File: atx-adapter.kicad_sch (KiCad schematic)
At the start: 1 part

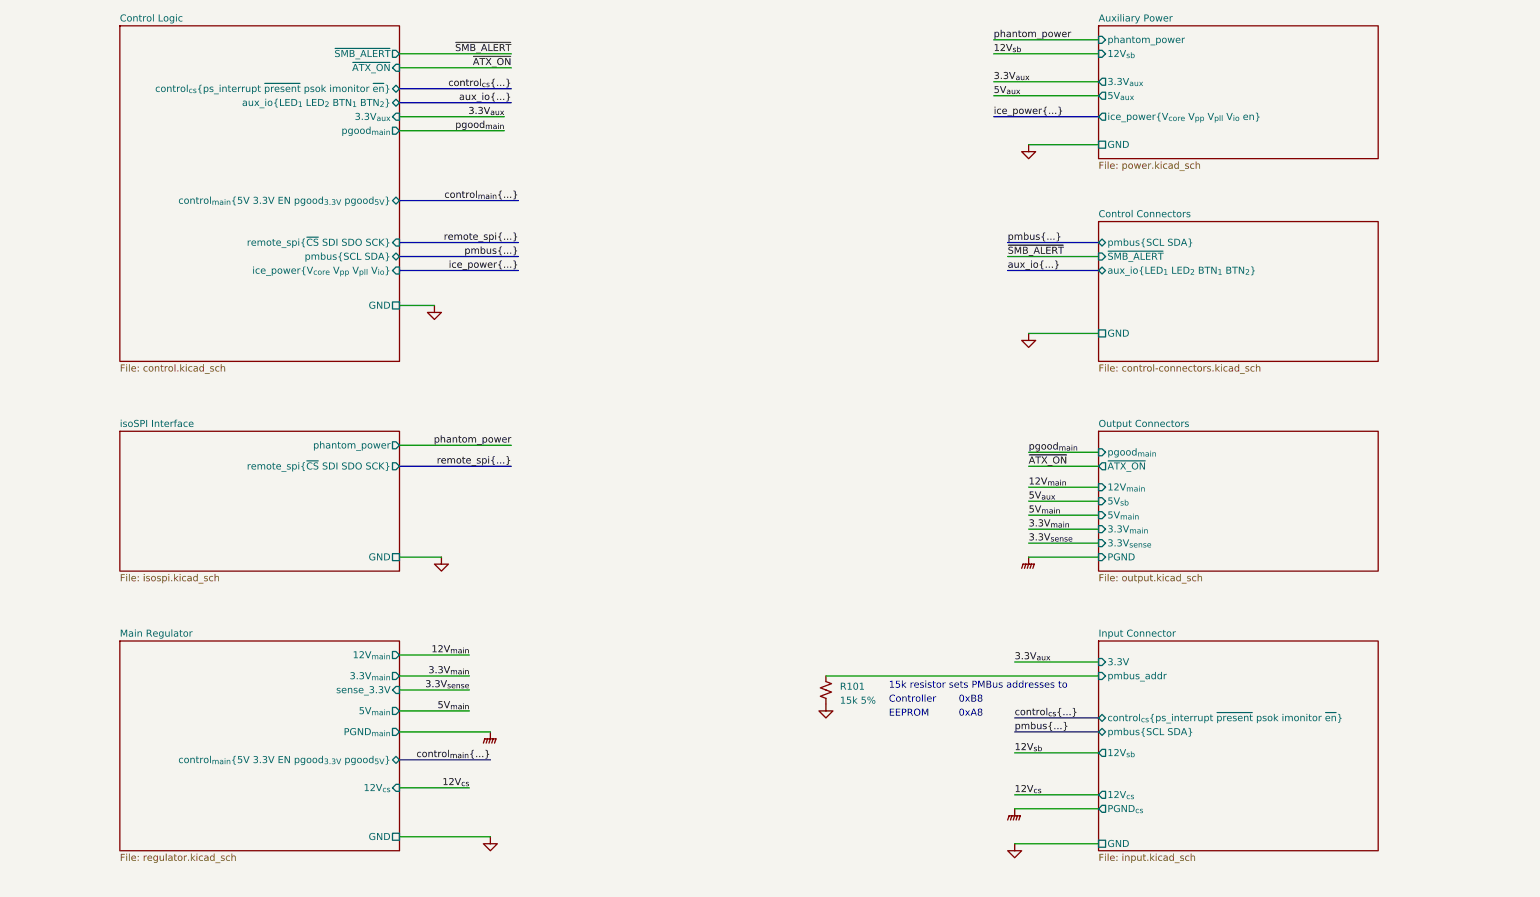
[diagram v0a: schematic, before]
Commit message: flesh out remote interface
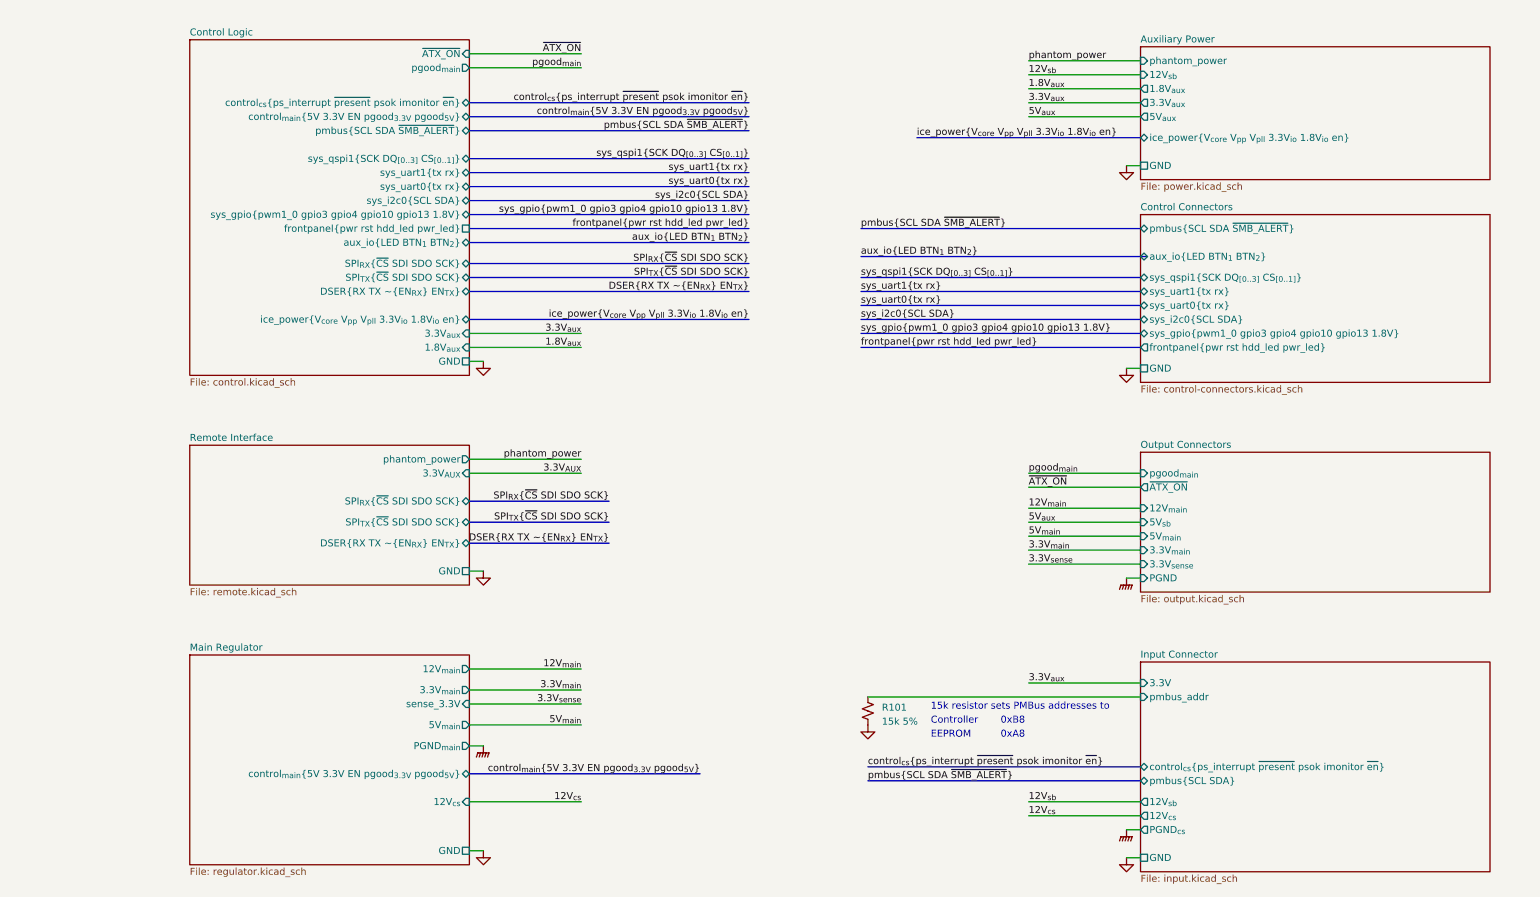
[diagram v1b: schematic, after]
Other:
- sheet isoSPI Interface renamed Remote Interface
- sheet Auxiliary Power ports: added 1.8V_{aux}, ice_power{V_{core} V_{pp} V_{pll} 3.3V_{io} 1.8V_{io} en}; removed ice_power{V_{core} V_{pp} V_{pll} V_{io} en}
- sheet Control Connectors ports: added aux_io{LED BTN_{1} BTN_{2}}, frontpanel{pwr rst hdd_led pwr_led}, pmbus{SCL SDA ~SMB_ALERT}, sys_gpio{pwm1_0 gpio3 gpio4 gpio10 gpio13 1.8V}, sys_i2c0{SCL SDA}, sys_qspi1{SCK DQ_{[0..3]} CS_{[0..1]}}, sys_uart0{tx rx}, sys_uart1{tx rx}; removed aux_io{LED_{1} LED_{2} BTN_{1} BTN_{2}}, pmbus{SCL SDA}, ~SMB_ALERT
- sheet Control Logic ports: added 1.8V_{aux}, DSER{RX TX ~EN_{RX} EN_{TX}}, SPI_{RX}{~CS SDI SDO SCK}, SPI_{TX}{~CS SDI SDO SCK}, aux_io{LED BTN_{1} BTN_{2}}, frontpanel{pwr rst hdd_led pwr_led}, ice_power{V_{core} V_{pp} V_{pll} 3.3V_{io} 1.8V_{io} en}, pmbus{SCL SDA ~SMB_ALERT}, sys_gpio{pwm1_0 gpio3 gpio4 gpio10 gpio13 1.8V}, sys_i2c0{SCL SDA}, sys_qspi1{SCK DQ_{[0..3]} CS_{[0..1]}}, sys_uart0{tx rx}, sys_uart1{tx rx}; removed aux_io{LED_{1} LED_{2} BTN_{1} BTN_{2}}, ice_power{V_{core} V_{pp} V_{pll} V_{io}}, pmbus{SCL SDA}, remote_spi{~CS SDI SDO SCK}, ~SMB_ALERT
- sheet Remote Interface: file isospi.kicad_sch -> remote.kicad_sch
- sheet Remote Interface ports: added 3.3V_{AUX}, DSER{RX TX ~EN_{RX} EN_{TX}}, SPI_{RX}{~CS SDI SDO SCK}, SPI_{TX}{~CS SDI SDO SCK}; removed remote_spi{~CS SDI SDO SCK}
- moved on the sheet: R101
